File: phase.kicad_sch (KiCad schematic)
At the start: 19 parts

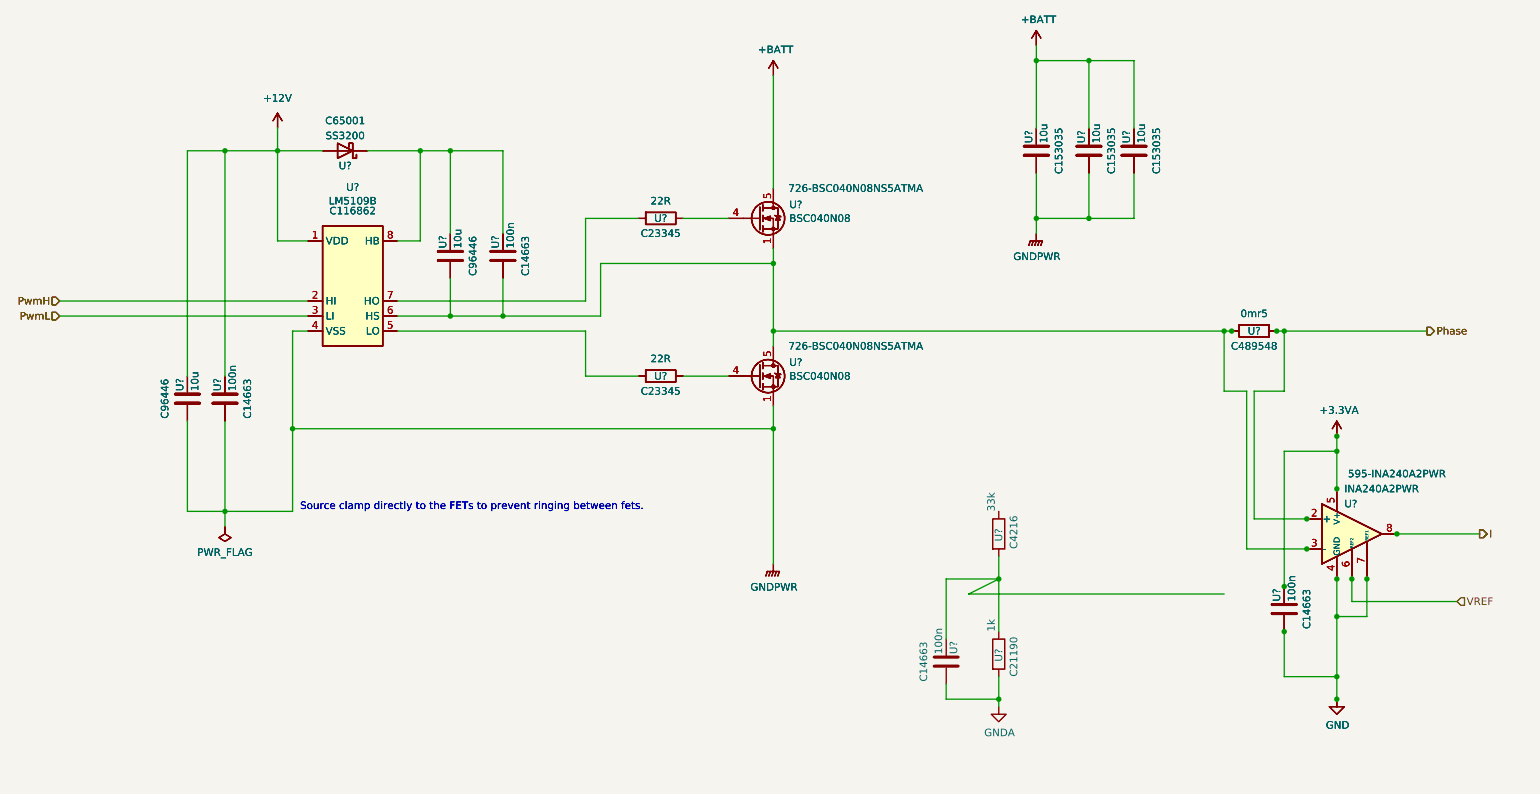
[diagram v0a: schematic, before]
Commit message: finished schematics
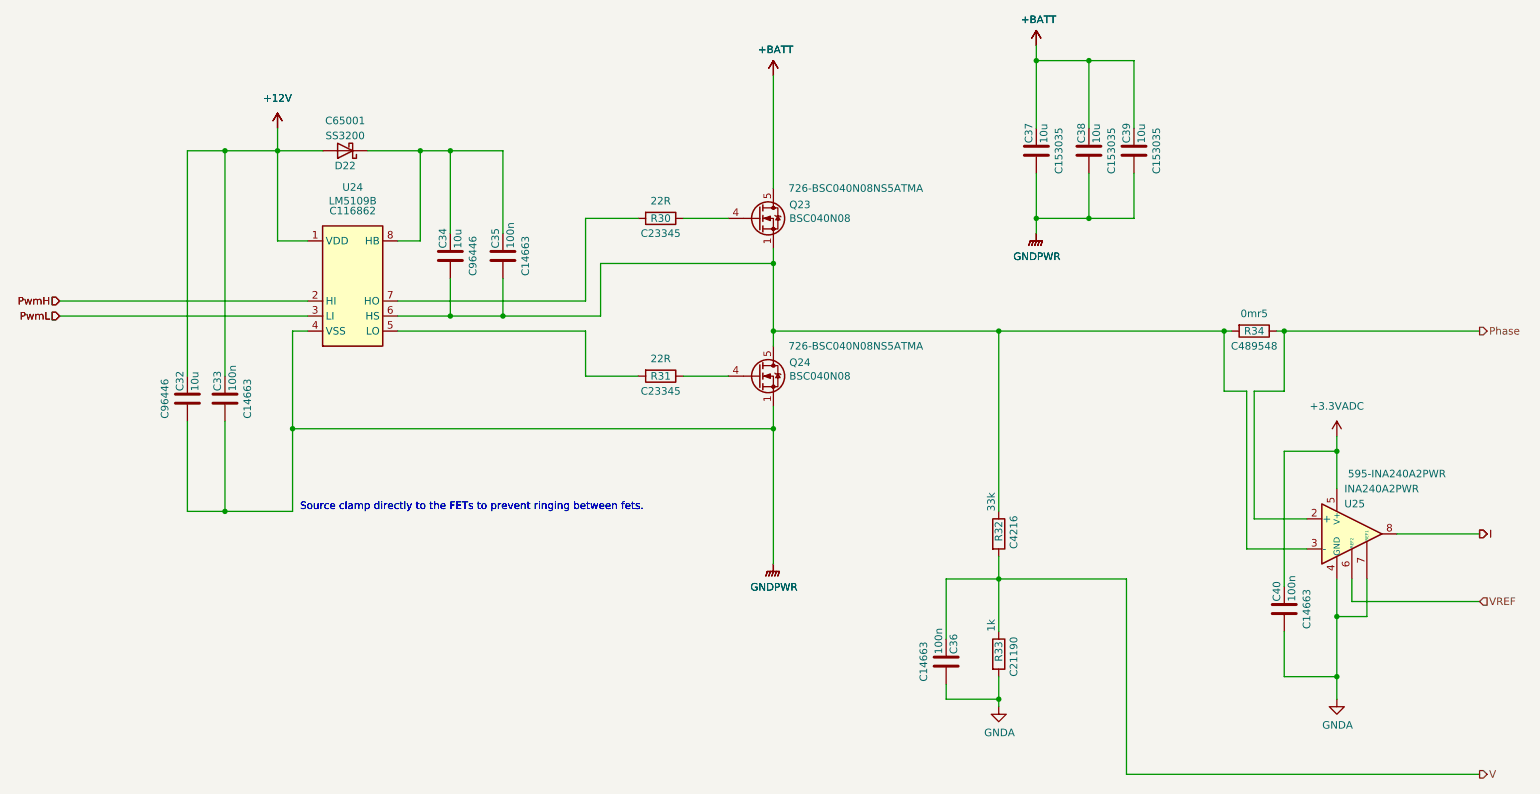
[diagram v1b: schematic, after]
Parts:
- removed U?: BSC040N08, Package_TO_SOT_SMD:LFPAK56_ThermalVias-1, symbol Transistor_FET:BSC040N08NS5
- removed U?: 22R, Resistor_SMD:R_0603_1608Metric, symbol Device:R
- removed U?: 0mr5, Resistor_SMD:R_2512_6332Metric, symbol Device:R
- removed U?: 10u, Capacitor_SMD:C_2220_5650Metric, symbol Device:C
- added C39: 10u, Capacitor_SMD:C_2220_5650Metric, symbol Device:C
- added Q24: BSC040N08, Package_TO_SOT_SMD:TDSON-8-1, symbol Transistor_FET:BSC040N08NS5
- added R31: 22R, Resistor_SMD:R_0603_1608Metric, symbol Device:R
- added R34: 0mr5, Resistor_SMD:R_2512_6332Metric, symbol Device:R
- Q23: renamed from U?; footprint Package_TO_SOT_SMD:LFPAK56_ThermalVias-1 -> Package_TO_SOT_SMD:TDSON-8-1
- gave numbers to parts that had none: 14
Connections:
- net GND is gone; now on net GNDA: C40.2, U25.1 (GND), U25.4 (GND), U25.7 (REF1)
- net +BATT: now also C39.1
- net GNDPWR: now also C39.2, Q24.1 (S), Q24.2 (S), Q24.3 (S)
- net Phase: now also R34.1
- net at C34.2, C35.2, Q23.1 (S)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: now also R32.1, Q24.5 (D), R34.2
- net at U24.5 (LO): now also R31.2
- net V: now reaches C36.1, R32.2, R33.1
- net +3.3VA renamed +3.3VADC
- new net: Q24.4 (G), R31.1
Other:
- company: (none) -> UNIMOC universal motor controller
- title: Phase -> (BCC) Battery Case Controller
